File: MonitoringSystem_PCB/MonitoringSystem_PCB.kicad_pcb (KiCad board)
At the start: 2 copper layers, 89 x 42 mm, 88 parts, among them IC1 MAX660M_NOPB, J1 Ultrasonic_Conn_2, J2 UJ2-BH-W1-TH, J3 Ultrasonic_Conn_1, J4 Conn_ARM_JTAG_SWD_10, J5 046288015000846+, Q1 SS8050-G, Q2 SS8050-G, SW1 SW_Push, SW2 SW_Push, U1 CP2102N-Axx-xQFN28, U10 OPA192IDBVR, U11 TDC1000PW, U2 ESP32-S3-WROOM-1-N16R2, U3 TDC7200PW, U5 OPA192IDBVR, U6 LM1117MP-3.3

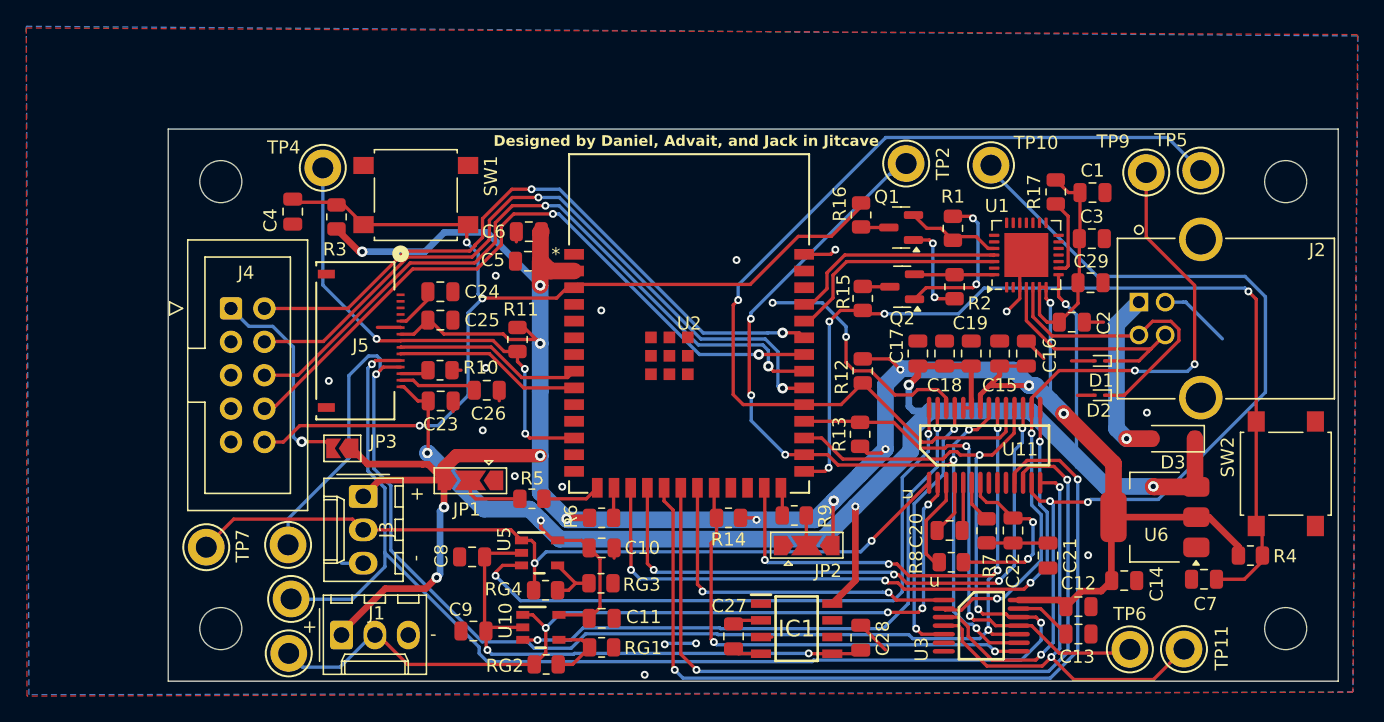
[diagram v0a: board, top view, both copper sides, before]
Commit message: most recent pcb
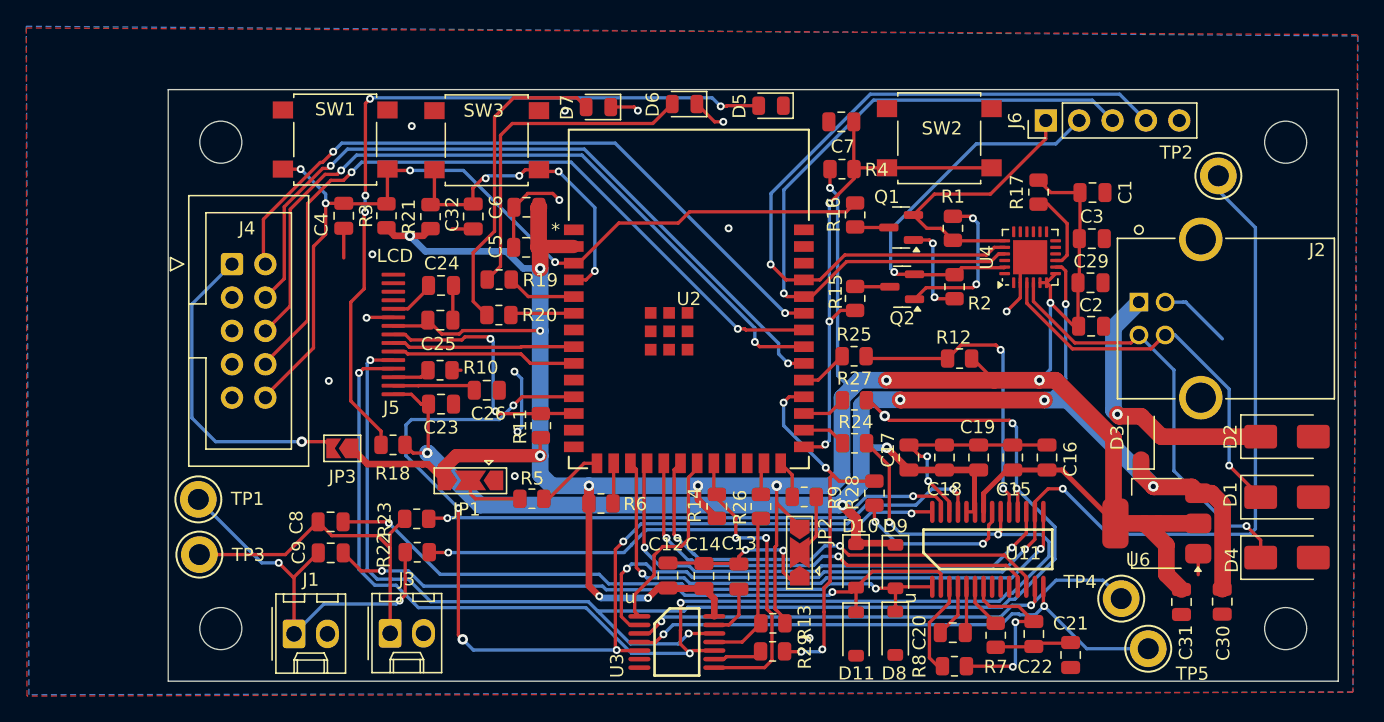
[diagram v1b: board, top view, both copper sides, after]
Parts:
- removed C10, C11: 0.1 uF, Capacitor_SMD:C_0805_2012Metric
- removed C27, C28: 10 uF, Capacitor_SMD:C_0805_2012Metric
- removed IC1: MAX660M_NOPB, MAX660:SOIC127P600X175-8N
- removed RG1, RG2, RG3, RG4: R, Resistor_SMD:R_0805_2012Metric
- removed TP10, TP11, TP6, TP7, TP8, TP9: TestPoint, TestPoint:TestPoint_Keystone_5010-5014_Multipurpose
- removed U1: CP2102N-Axx-xQFN28, Package_DFN_QFN:QFN-28-1EP_5x5mm_P0.5mm_EP3.35x3.35mm
- removed U10, U5: OPA192IDBVR, OPA192IDBVR Amp:DBV0005A_N
- added C30: 10 uF, Capacitor_SMD:C_0805_2012Metric, F.Cu at (191.2, 119.0)
- added C31: 10 uF, Capacitor_SMD:C_0805_2012Metric, F.Cu at (188.1, 119.0)
- added C32: 1 uF, Capacitor_SMD:C_0805_2012Metric, F.Cu at (134.2, 89.7)
- added D10: MBR0520, Diode_SMD:D_SOD-123, F.Cu at (163.3, 116.2)
- added D11: MBR0520, Diode_SMD:D_SOD-123, F.Cu at (163.3, 121.4)
- added D4: SMAJ5.0CA, Diode_SMD:D_SMA, F.Cu at (196.1, 115.6)
- added D5: PWR_IND, LED_SMD:LED_0805_2012Metric, F.Cu at (156.8, 81.2)
- added D6: PAIR_IND, LED_SMD:LED_0805_2012Metric, F.Cu at (150.3, 81.1)
- added D7: CONN_IND, LED_SMD:LED_0805_2012Metric, F.Cu at (143.7, 81.3)
- added D8: MBR0520, Diode_SMD:D_SOD-123, F.Cu at (166.3, 121.4)
- added D9: MBR0520, Diode_SMD:D_SOD-123, F.Cu at (166.3, 116.3)
- added J6: Conn_01x05_Female, Connector_PinHeader_2.54mm:PinHeader_1x05_P2.54mm_Vertical, F.Cu at (177.8, 82.3)
- added R18: 1k, Resistor_SMD:R_0805_2012Metric, F.Cu at (128.1, 107.0)
- added R19: 1k, Resistor_SMD:R_0805_2012Metric, F.Cu at (136.2, 94.5)
- added R20: 1k, Resistor_SMD:R_0805_2012Metric, F.Cu at (136.2, 97.2)
- added R21: 100k, Resistor_SMD:R_0805_2012Metric, F.Cu at (130.9, 89.7)
- added R22: TRACE_MATCH, Resistor_SMD:R_0805_2012Metric, F.Cu at (129.9, 115.2)
- added R23: TRACE_MATCH, Resistor_SMD:R_0805_2012Metric, F.Cu at (129.9, 112.7)
- added R24: SPI_R, Resistor_SMD:R_0805_2012Metric, F.Cu at (163.2, 106.9)
- added R25: SPI_R, Resistor_SMD:R_0805_2012Metric, F.Cu at (163.2, 100.3)
- added R26: SPI_R, Resistor_SMD:R_0805_2012Metric, F.Cu at (156.1, 111.7)
- added R27: SPI_R, Resistor_SMD:R_0805_2012Metric, F.Cu at (163.2, 103.6)
- added R28: SPI_R, Resistor_SMD:R_0805_2012Metric, F.Cu at (164.7, 110.7)
- added R29: SPI_R, Resistor_SMD:R_0805_2012Metric, F.Cu at (157.0, 122.7)
- added SW3: SW_Push, Button_Switch_SMD:SW_SPST_B3S-1000, F.Cu at (135.2, 83.8)
- added U4: CP2102N-Axx-xQFN24, Package_DFN_QFN:QFN-24-1EP_4x4mm_P0.5mm_EP2.6x2.6mm, F.Cu at (176.6, 92.8)
- C1: value 1.0 uF -> 1 uF
- C20: value C -> 1 nF
- C21: value C -> 53 pF
- C22: value C -> 50 pF
- C4, C7: value 1u -> 1 uF
- C8, C9: value 0.1 uF -> RX_GAIN
- D1, D2: value SZESD9B5.0ST5G -> SMAJ5.0CA; footprint Diode_SMD:D_SOD-923 -> Diode_SMD:D_SMA
- J1: value Ultrasonic_Conn_2 -> Conn_01x02; footprint Connector_Molex:Molex_KK-254_AE-6410-03A_1x03_P2.54mm_Vertical -> Connector_Molex:Molex_KK-254_AE-6410-02A_1x02_P2.54mm_Vertical
- J3: value Ultrasonic_Conn_1 -> Conn_01x02; footprint Connector_Molex:Molex_KK-254_AE-6410-03A_1x03_P2.54mm_Vertical -> Connector_Molex:Molex_KK-254_AE-6410-02A_1x02_P2.54mm_Vertical
- J5: footprint ZIF_LCD_connector:CONN15_6288_7X5P7_AVX -> ZIF_LCD_connector:15Pin_TAB
- R7: value R -> 1k
- R8: value R -> 5k
- moved TP4 69.0 mm to (183.5, 118.7)
- moved C7 44.4 mm to (162.2, 82.5)
- moved R4 42.8 mm to (162.2, 86.0)
- moved SW2 36.7 mm to (169.7, 83.7), turned to 0 degrees
- moved TP5 36.6 mm to (185.5, 122.5)
- moved C14 32.0 mm to (151.8, 117.0), turned to 90 degrees
- moved C12 31.3 mm to (149.0, 117.0), turned to 90 degrees
- moved C13 26.2 mm to (154.4, 117.0), turned to 90 degrees
- moved TP2 23.8 mm to (190.9, 86.6)
- moved U3 23.2 mm to (149.7, 122.0)
- moved D1 17.6 mm to (196.1, 111.0), turned to 0 degrees
- moved R13 15.8 mm to (157.0, 120.6), turned to 0 degrees
- moved D2 14.6 mm to (196.1, 106.4), turned to 0 degrees
- moved C9 12.4 mm to (123.4, 115.2), turned to 0 degrees
- moved C8 11.1 mm to (123.3, 112.9), turned to 0 degrees
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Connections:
- net Net-(Q1-E) renamed /Power and Programming Subsystem/RTS
- net Net-(Q2-E) renamed /Power and Programming Subsystem/DTR
- C8 pad 1: -5V -> /Ultrasonic Sensing Subsystem/ULTRASONIC_2
- C8 pad 2: GND -> /Ultrasonic Sensing Subsystem/SENSOR_RX_1
- C9 pad 1: -5V -> /Ultrasonic Sensing Subsystem/ULTRASONIC_1
- C9 pad 2: GND -> /Ultrasonic Sensing Subsystem/SENSOR_RX_2
- D2 pad 1: /Power and Programming Subsystem/USB_D- -> Net-(D2-A1)
- D3 pad 2: Net-(D3-A) -> Net-(D2-A1)
- J1 pad 1: +3.3V -> /Ultrasonic Sensing Subsystem/ULTRASONIC_1
- J1 pad 2: /Ultrasonic Sensing Subsystem/ULTRASONIC_2_IN -> GND
- J2 pad 1: Net-(D3-A) -> Net-(D2-A1)
- J3 pad 1: +3.3V -> /Ultrasonic Sensing Subsystem/ULTRASONIC_2
- J3 pad 2: /Ultrasonic Sensing Subsystem/ULTRASONIC_1_IN -> GND
- TP1 pad 1: SPI_MOSI -> /Ultrasonic Sensing Subsystem/ULTRASONIC_1
- TP2 pad 1: SPI_MISO -> /Ultrasonic Sensing Subsystem/TRIGGER
- TP3 pad 1: SPI_SCK -> /Ultrasonic Sensing Subsystem/ULTRASONIC_2
- TP4 pad 1: /LCD_CS -> /Ultrasonic Sensing Subsystem/START
- TP5 pad 1: TDC1000_CS -> /Ultrasonic Sensing Subsystem/STOP
- U11 pad 1: /Ultrasonic Sensing Subsystem/ULTRASONIC_1_IN -> /Ultrasonic Sensing Subsystem/SENSOR_RX_1
- U11 pad 2: /Ultrasonic Sensing Subsystem/ULTRASONIC_2_IN -> /Ultrasonic Sensing Subsystem/SENSOR_RX_2
- U11 pad 21: SPI_MISO -> Net-(U11-SDO)
- U11 pad 27: /Ultrasonic Sensing Subsystem/TRANSMIT_2_OUT -> /Ultrasonic Sensing Subsystem/TX_SIGNAL_2
- U11 pad 28: /Ultrasonic Sensing Subsystem/TRANSMIT_1_OUT -> /Ultrasonic Sensing Subsystem/TX_SIGNAL_1
- U2 pad 11: CLK_OUT3 (8 MHz) -> CLK_OUT3 (1 MHz)
- U2 pad 25: SPI_MOSI -> Net-(U2-IO48)
- U2 pad 28: SPI_MISO -> Net-(U2-IO35)
- U2 pad 29: SPI_SCK -> Net-(U2-IO36)
- U2 pad 30: TDC7200_CS -> SPI_MISO
- U2 pad 31: TDC1000_CS -> Net-(U2-IO38)
- U2 pad 4: unconnected-(U2-IO4-Pad4) -> /SOFT_RST
- U2 pad 5: unconnected-(U2-IO5-Pad5) -> /PAIR_IND
- U2 pad 6: unconnected-(U2-IO6-Pad6) -> /CONN_IND
- U3 pad 9: SPI_MISO -> Net-(U3-DOUT)
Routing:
- net /Ultrasonic Sensing Subsystem/ULTRASONIC_2_IN: track 65.6 -> 0.00 mm, vias 4 -> 0
- net /Ultrasonic Sensing Subsystem/ULTRASONIC_1_IN: track 62.8 -> 0.00 mm, vias 2 -> 0
- net CLK_OUT3 (1 MHz): track 20.4 -> 82.7 mm, vias 2 -> 6
- net Net-(D5-A): track 0.00 -> 57.8 mm, vias 0 -> 4
- net TDC1000_CS: track 75.1 -> 23.5 mm, vias 1 -> 2
- net /Ultrasonic Sensing Subsystem/SENSOR_RX_2: track 0.00 -> 50.5 mm, vias 0 -> 2
- net /Ultrasonic Sensing Subsystem/SENSOR_RX_1: track 0.00 -> 49.3 mm, vias 0 -> 2
- net /Ultrasonic Sensing Subsystem/TRANSMIT_1_OUT: track 49.3 -> 0.00 mm, vias 2 -> 0
- net /Ultrasonic Sensing Subsystem/TRANSMIT_2_OUT: track 46.3 -> 0.00 mm, vias 2 -> 0
- net -5V: track 42.0 -> 0.00 mm, vias 2 -> 0
- net /Ultrasonic Sensing Subsystem/TX_SIGNAL_2: track 0.00 -> 40.6 mm, vias 0 -> 2
- net RX: track 16.8 -> 57.2 mm, vias 0 -> 1
- net /Ultrasonic Sensing Subsystem/TX_SIGNAL_1: track 0.00 -> 39.6 mm, vias 0 -> 2
- net TX: track 17.3 -> 54.6 mm, vias 0 -> 1
- net /Ultrasonic Sensing Subsystem/TRIGGER: track 51.3 -> 87.9 mm, vias 4 -> 3
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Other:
- board size 89 x 42 mm -> 89 x 45 mm
